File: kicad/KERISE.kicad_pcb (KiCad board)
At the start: 2 copper layers, 40 x 44.5 mm, 119 parts, among them J1 Host, J2 Slave, J3 Host, J4 Slave, J5 COM, J6 Host, J7 Slave, J8 Host, J9 Slave, P1 Motor_L, P10 ENC_Slave, P2 Motor_R, P3 Battery, P4 Fan, P5 ENC_Host, P6 ENC_Slave, P7 ToF_Host, P8 ToF_Slave, P9 ENC_Host, Q1 DMN3065LW-7, Q2 DMN3065LW-7, Q3 DMN3065LW-7, Q4 DMN3065LW-7, Q5 DMN3065LW-7, SW1 SW_Push, SW2 SW_Push, U1 ESP32, U10 TLV316IDCKR, U11 TLV316IDCKR, U12 ICM-20602, U13 PCA9632, U14 LMV321, U2 DRV8835, U3 LXDC2URxx, U4 TLV316IDCKR, U5 TLV316IDCKR, U6 AS5048A, U7 VL53L0X, U8 AS5048A, U9 ICM-20602

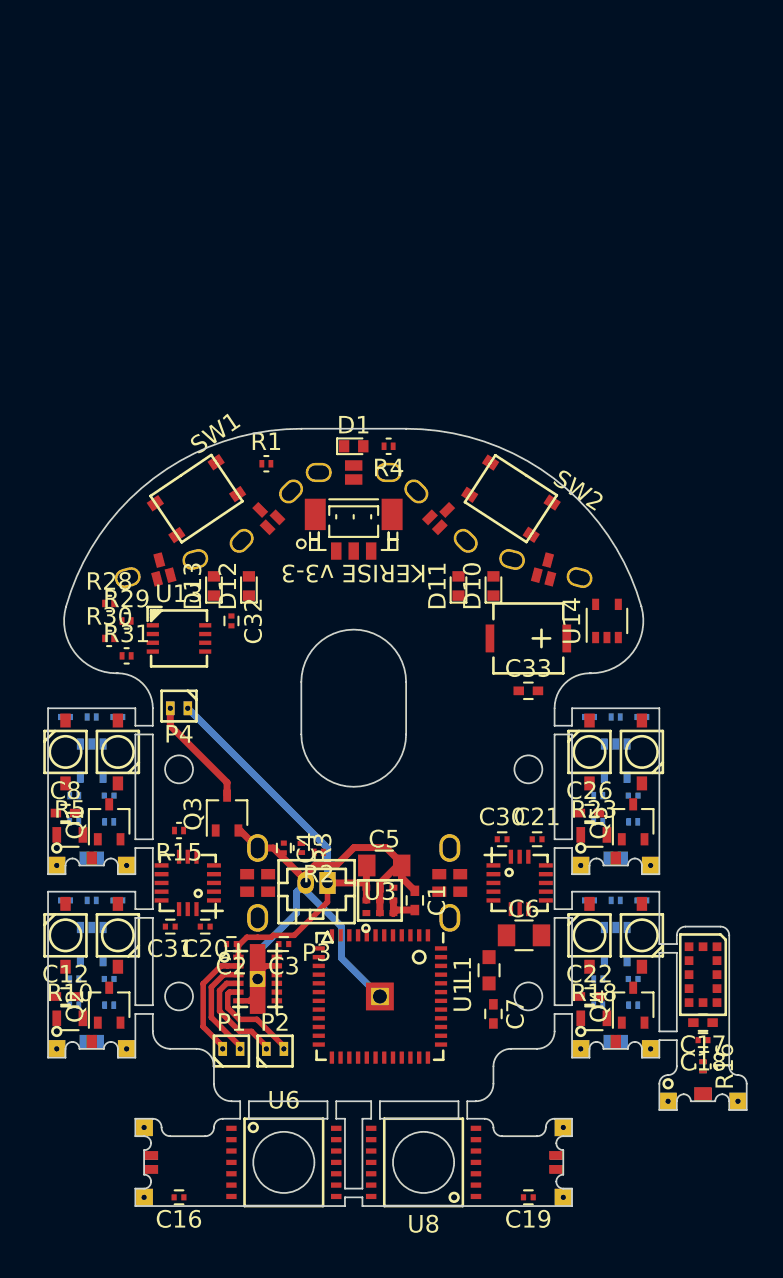
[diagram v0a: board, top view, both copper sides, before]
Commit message: 自動配線成功
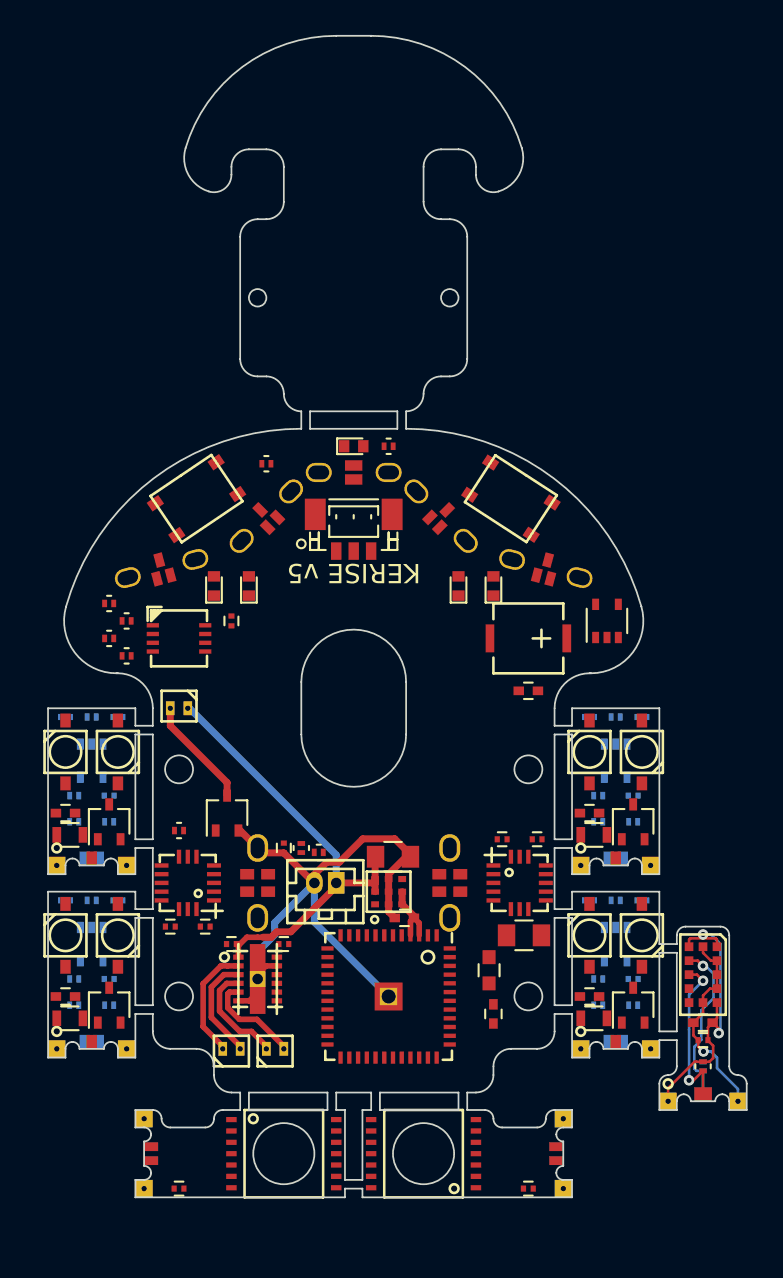
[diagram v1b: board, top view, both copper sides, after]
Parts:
- P3: footprint Connectors_Hirose:Hirose_DF13-02P-1.25DSA_02x1.25mm_Straight -> mouse:Hirose_DF13-02P-1.25DSA_02x1.25mm_Straight
- moved C11 3.00 mm to (132.0, 103.5), turned to 0 degrees
- moved C9 3.00 mm to (135.0, 103.5), turned to 180 degrees
- moved C1 1.17 mm to (151.4, 115.0), turned to 0 degrees
- moved C5 0.71 mm to (150.8, 111.5)
- moved U3 0.71 mm to (150.5, 113.5)
- moved C16 0.50 mm to (138.5, 130.5)
- moved C19 0.50 mm to (158.5, 130.5)
- moved P10 0.50 mm to (160.5, 128.5)
- moved P3 0.50 mm to (147.5, 113.0)
- moved P6 0.50 mm to (136.5, 128.5)
- moved U1 0.50 mm to (150.5, 119.5)
- moved U6 0.50 mm to (144.5, 128.5)
- moved U8 0.50 mm to (152.5, 128.5)
- turned R6 to 180 degrees
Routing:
- net /ToF/s_3.3V: track 0.00 -> 17.4 mm, vias 0 -> 2
- net /ToF/s_GND: track 0.00 -> 11.5 mm, vias 0 -> 1
- net /ToF/s_SCL: track 0.00 -> 9.49 mm, vias 0 -> 1
- net /ToF/s_SDA: track 0.00 -> 9.34 mm, vias 0 -> 2
- net +3V3: track 2.06 -> 3.99 mm
- net +BATT: track 25.6 -> 26.3 mm
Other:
- board size 40 x 44.5 mm -> 40 x 66.5 mm
- net class 3.3V: trace_width 0.16 -> 0.18; via_dia 0.5 -> 0.6
- net class Analog: via_dia 0.5 -> 0.6
- net class Antena: clearance 0.18 -> 0.15; trace_width 0.18 -> 0.2; via_dia 0.5 -> 0.6
- net class BATT: via_dia 0.5 -> 0.6
- net class Default: via_dia 0.5 -> 0.6
- net class GND: trace_width 0.16 -> 0.18; via_dia 0.5 -> 0.6
- net class LED: via_dia 0.5 -> 0.6
- net class Motor: via_dia 0.5 -> 0.6
- board text added: "KERISE v5"
- board text removed: "KERISE v3-3"
